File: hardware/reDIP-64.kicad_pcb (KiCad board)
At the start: 6 copper layers, 25.4 x 50.8 mm, 150 parts, among them J1 USB4080, J2 Conn_02x20_Counter_Clockwise, J3 Conn_01x20, J4 Conn_02x20_Odd_Even, J5 Conn_02x05_Odd_Even, Q1 PDTA143ZMB, SW1 KXT311LHS, U1 PTN5110NHQ, U10 FPF2495C, U11 TPS22916CN, U12 FAN53611, U13 NCP163AMX120TBG, U14 NCP115AMX250TCG, U15 NCP163AMX330TBG, U16 NCP163AMX120TBG, U17 SN74CBT16211ADGVR, U18 SN74CBT16211ADGVR, U19 SN74CBT16211ADGVR, U2 LFE5UM5G-25F-8MG285C, U20 SN74CBT16211ADGVR, U21 W957A8MFYA5I, U22 W25Q128JVPIM, U23 SGTL5000XNLA3, U3 FUSB340, U4 DSC1103CE2-135.0000, U5 FSUSB42UMX, U6 FPF2286, U7 FPF1048, U8 TPS22916CN, U9 FAN53610

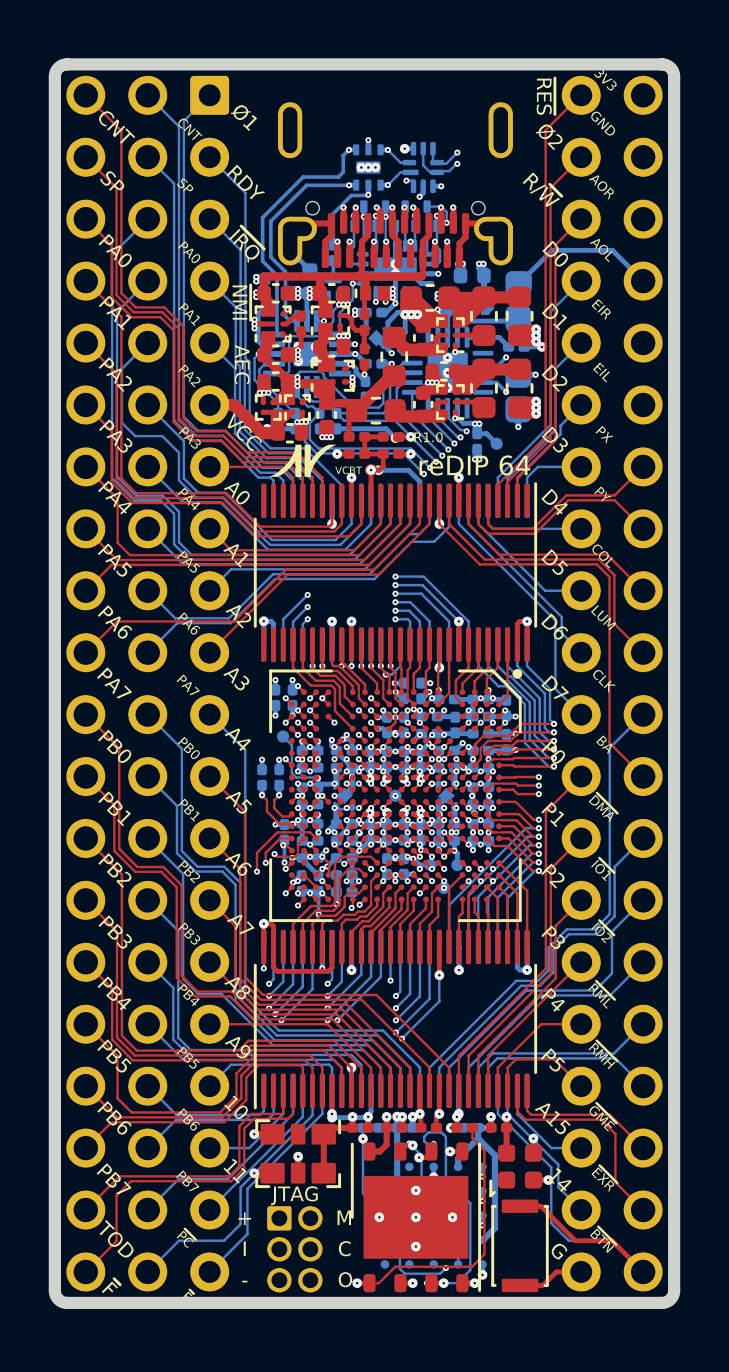
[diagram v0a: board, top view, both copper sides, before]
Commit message: Updated to KiCad 7
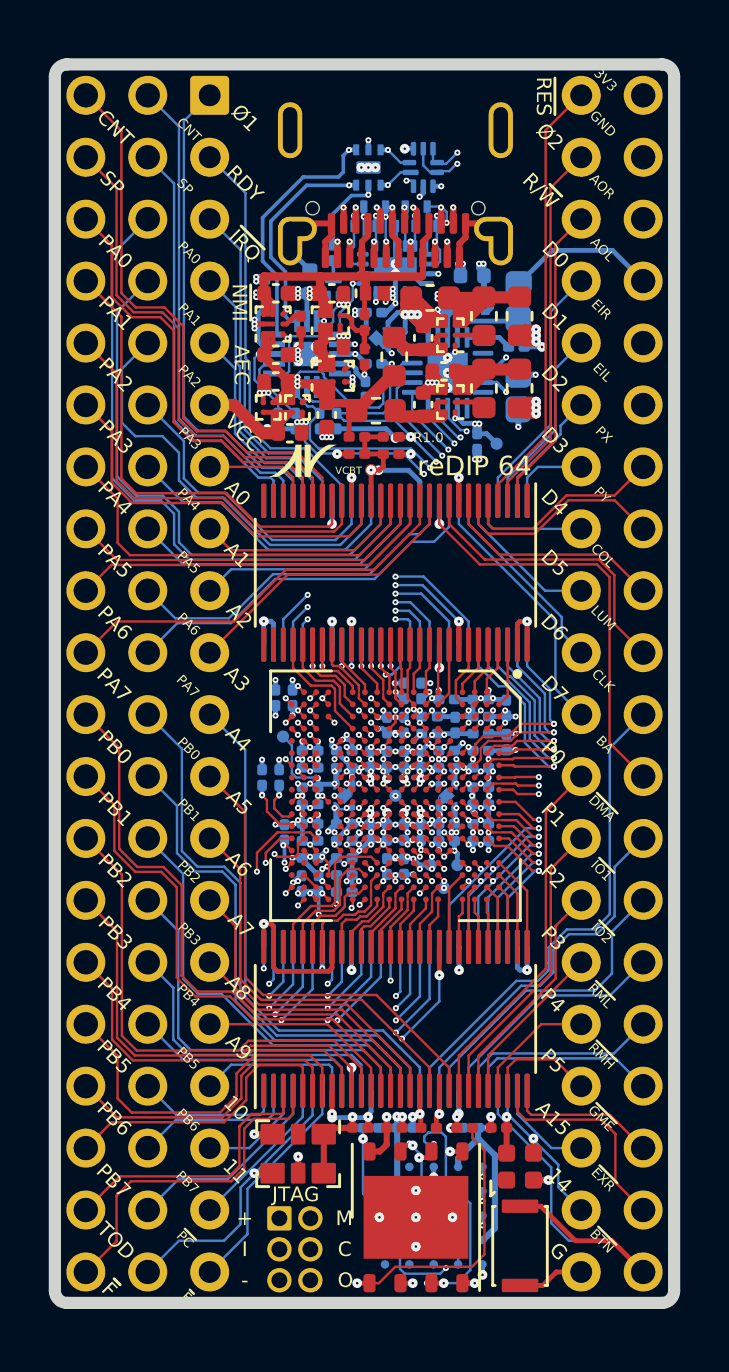
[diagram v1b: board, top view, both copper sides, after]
